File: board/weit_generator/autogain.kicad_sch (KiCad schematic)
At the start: 19 parts, among them Q1 BC547

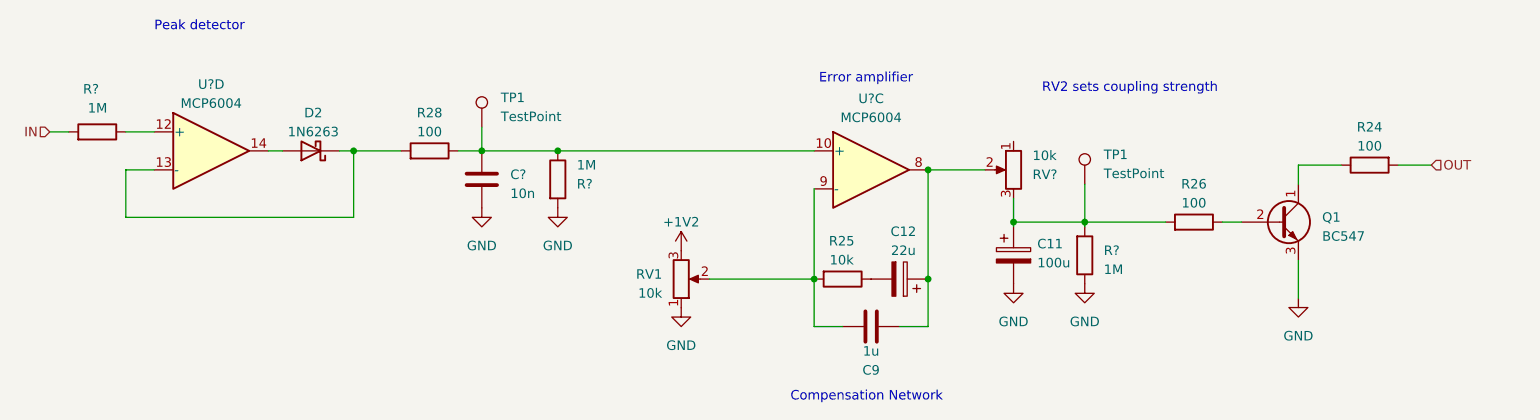
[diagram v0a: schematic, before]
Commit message: .
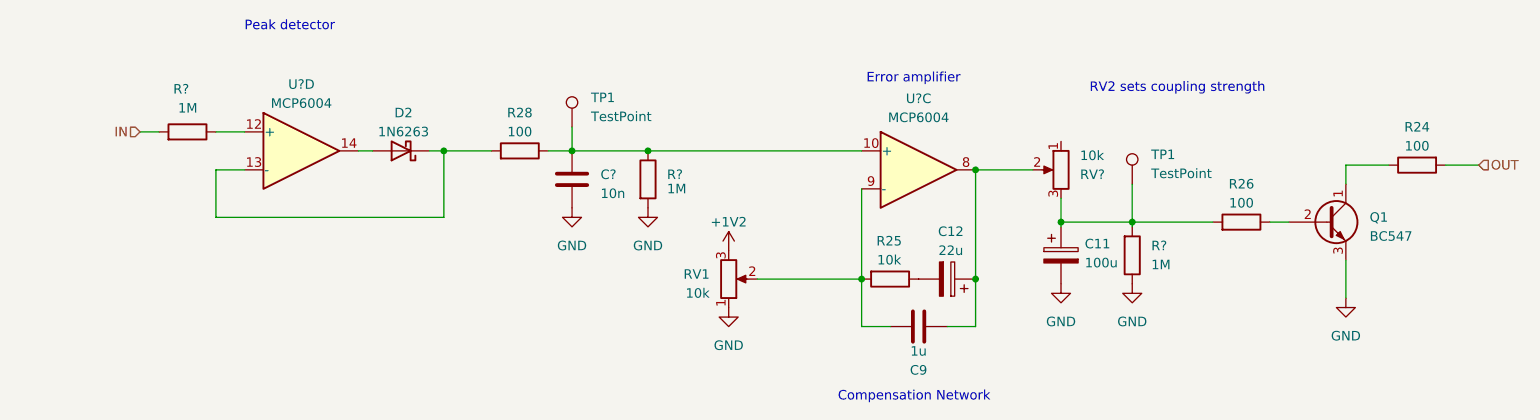
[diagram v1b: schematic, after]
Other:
- moved on the sheet: C11, C12, C9, C?, D2, Q1, R24, R25, R26, R28, R?, RV1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
